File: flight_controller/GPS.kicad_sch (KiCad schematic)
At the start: 25 parts, among them CN1 A1251WV-S-6P, CN2 A1251WV-S-4P, CN3 A1251WV-S-3P, J15 A1257WV-S-6P-LCP, J16 HCZZ0494-2, Q1 AO3400A

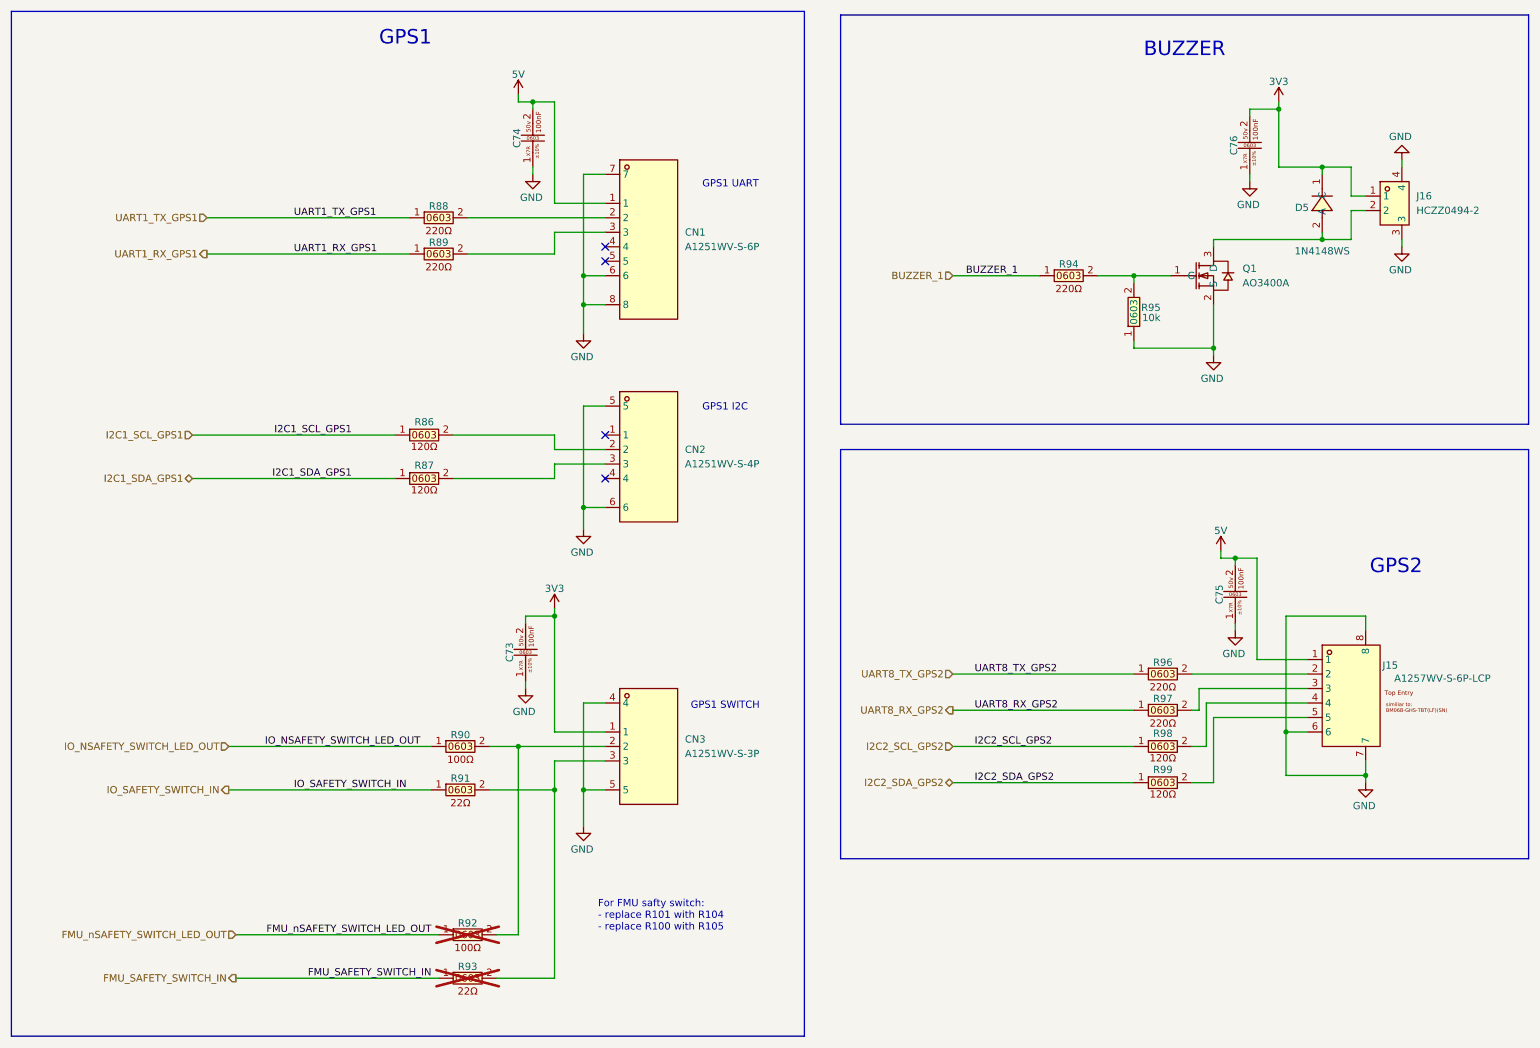
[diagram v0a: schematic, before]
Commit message: Updated power and usb connectors, annotations and netlist check
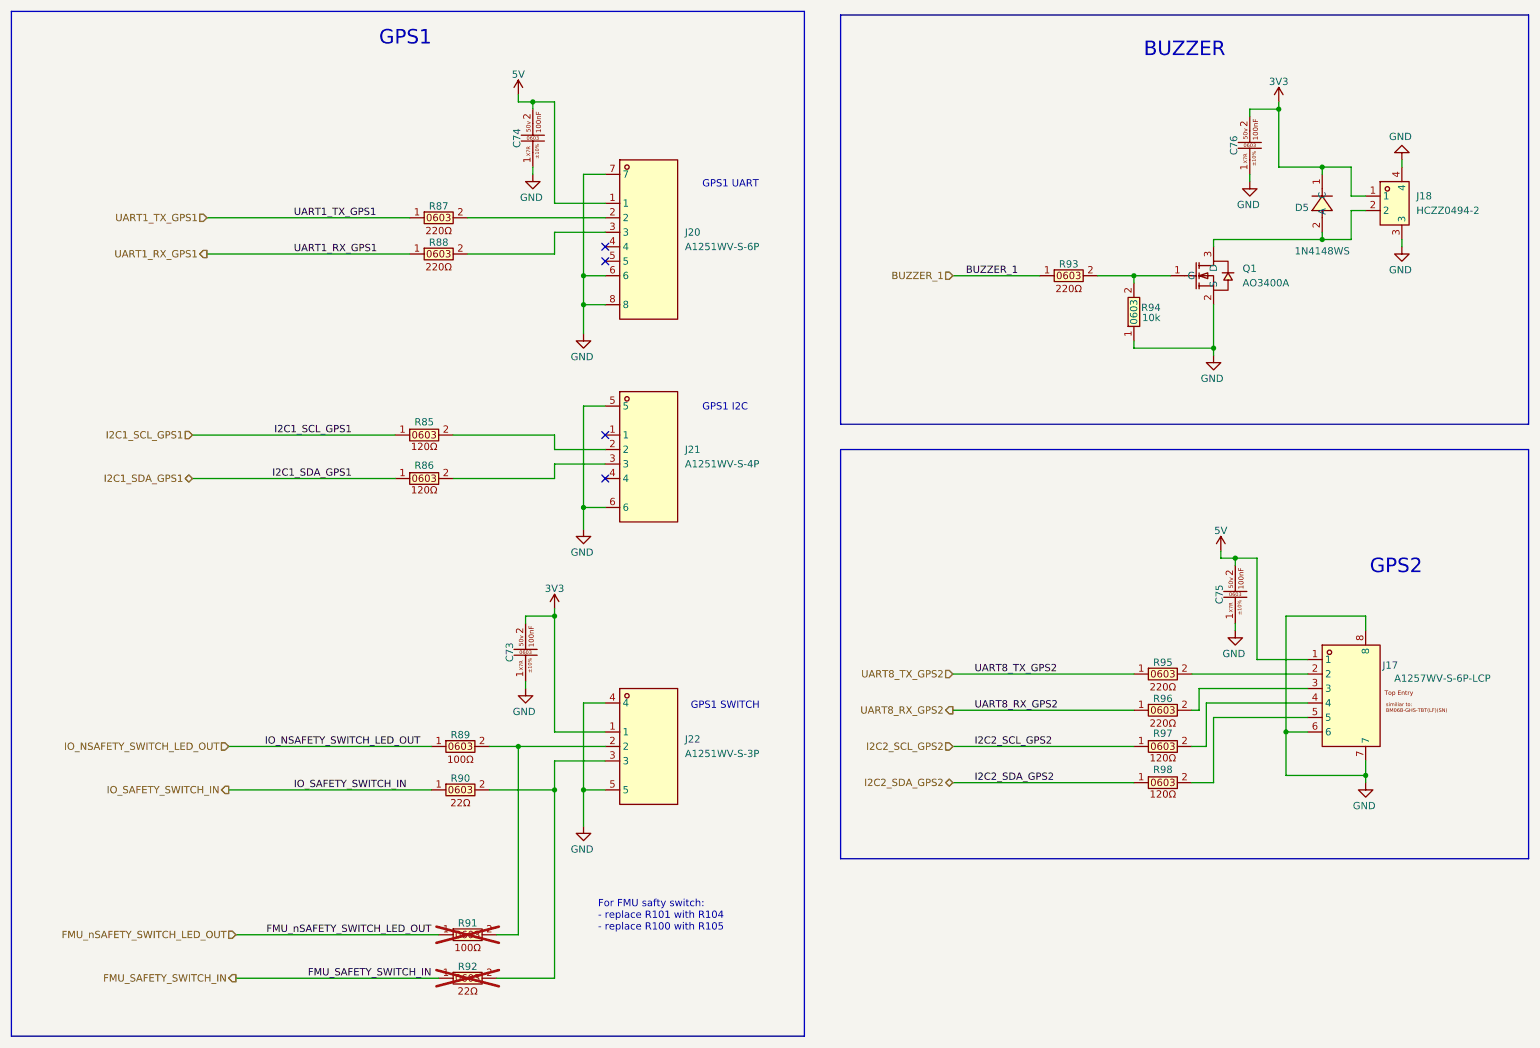
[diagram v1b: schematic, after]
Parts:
- renumbered J15 to J17, J16 to J18, CN1 to J20, CN2 to J21, CN3 to J22, R86 to R85, R87 to R86, R88 to R87, R89 to R88, R90 to R89, R91 to R90, R92 to R91, R93 to R92, R94 to R93, R95 to R94, R96 to R95, R97 to R96, R98 to R97, R99 to R98

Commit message: Revert to state of commit 2458262 moved all to components to top
Reverts commits: d012532, 3d9c600, 58bc0ac
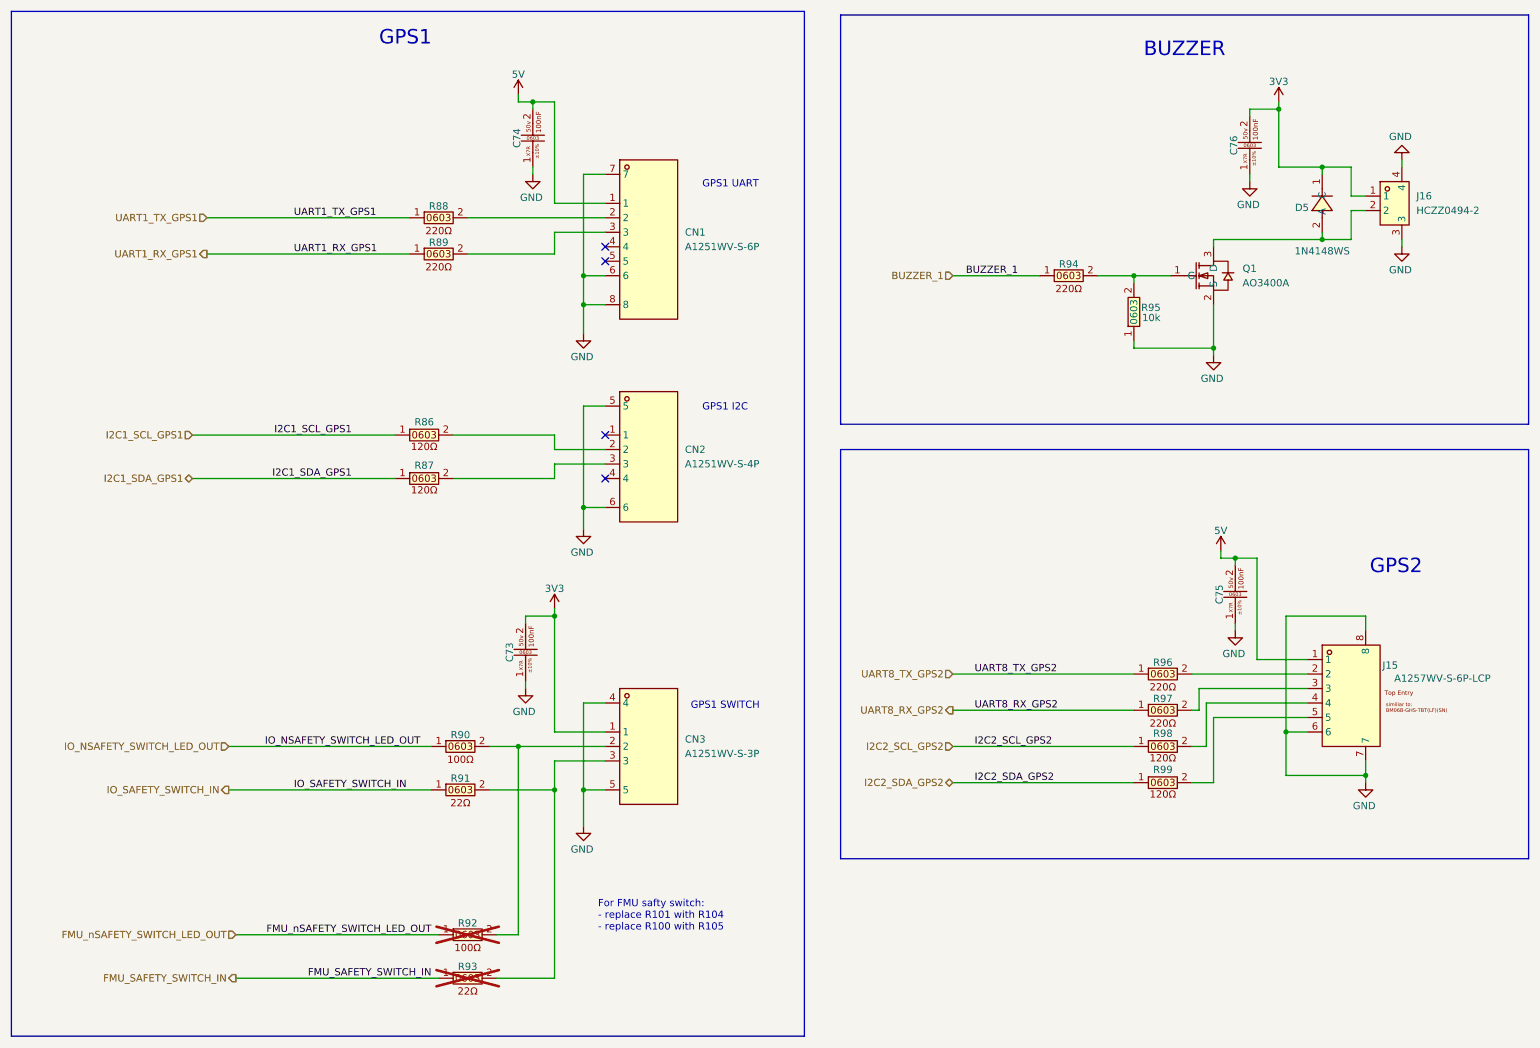
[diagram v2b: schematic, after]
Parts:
- renumbered J20 to CN1, J21 to CN2, J22 to CN3, J17 to J15, J18 to J16, R85 to R86, R86 to R87, R87 to R88, R88 to R89, R89 to R90, R90 to R91, R91 to R92, R92 to R93, R93 to R94, R94 to R95, R95 to R96, R96 to R97, R97 to R98, R98 to R99
